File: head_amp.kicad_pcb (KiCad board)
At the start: 2 copper layers, 42 x 64.5 mm, 26 parts, among them J1 Conn_01x02, J2 Headset Port, J3 Ear Mic Input, J4 Speaker Output, SW1 SW_Wuerth_450301014042, U1 LM124DR

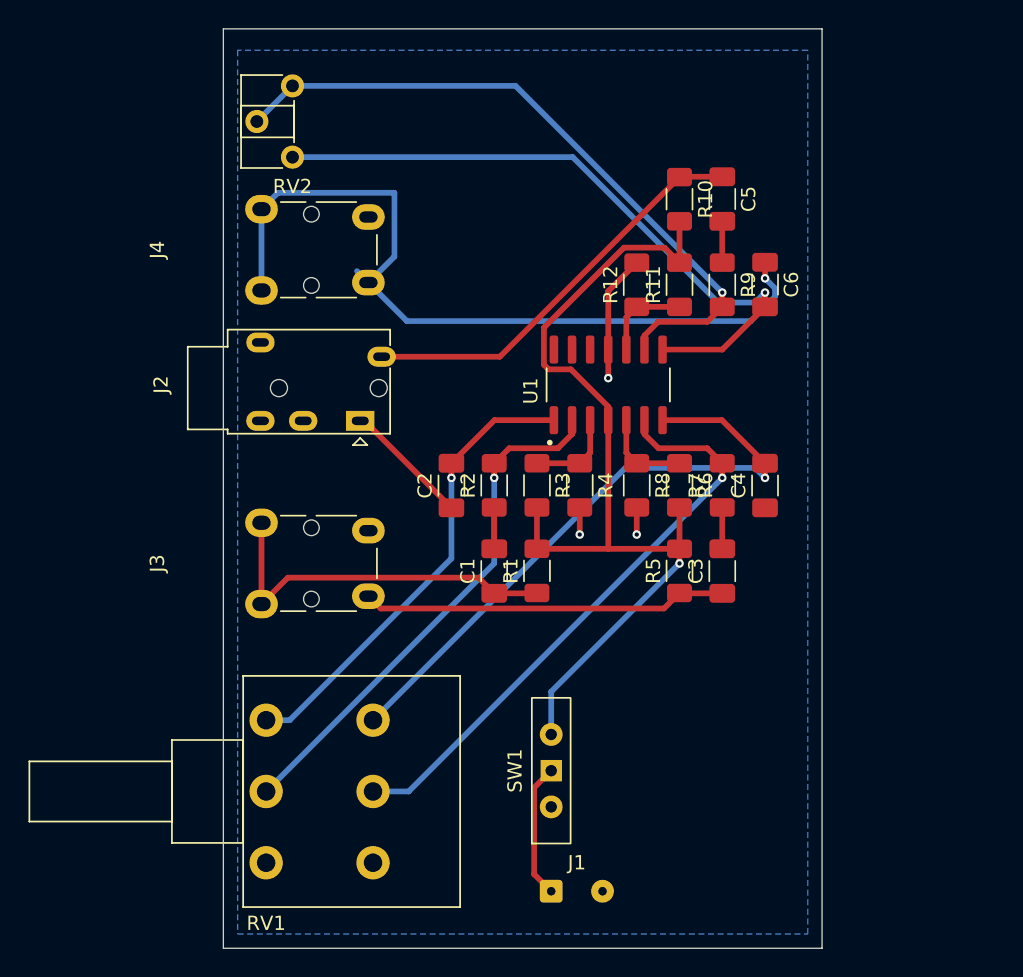
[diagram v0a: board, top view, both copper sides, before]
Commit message: Route PCB :3
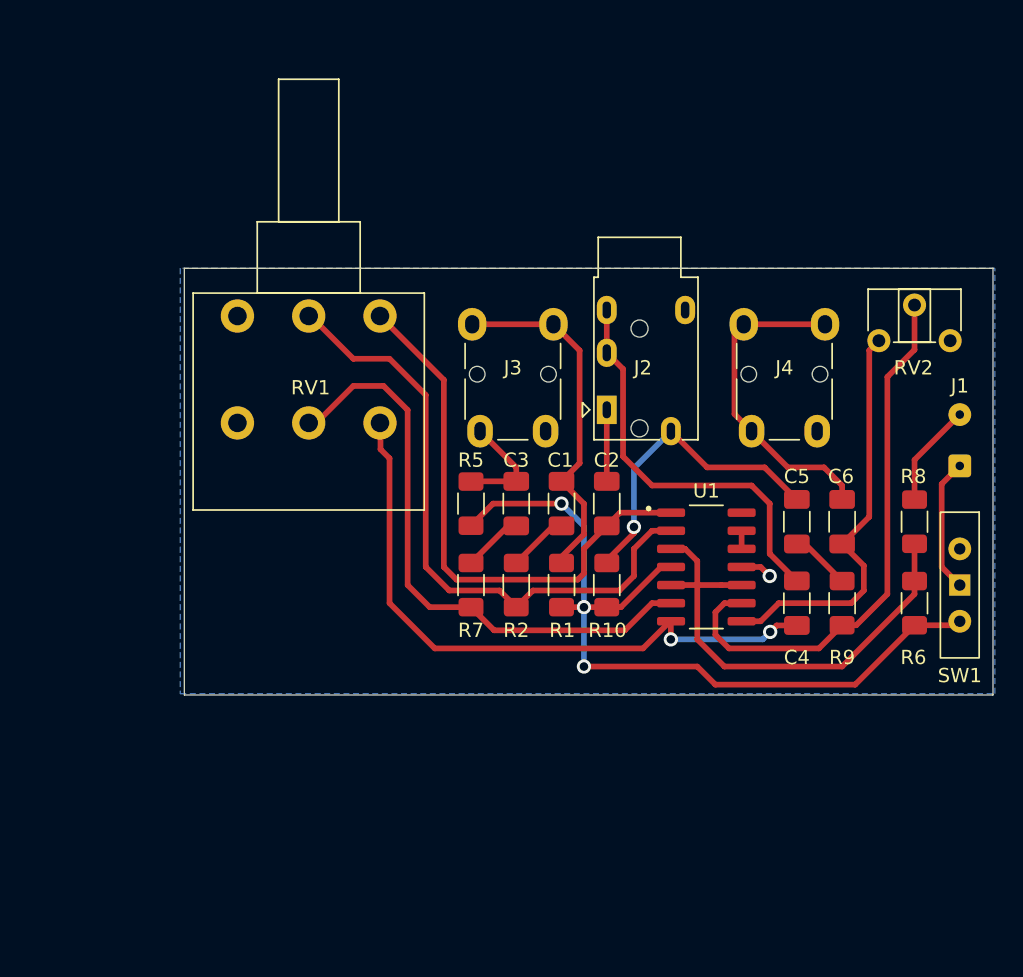
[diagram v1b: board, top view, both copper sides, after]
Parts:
- removed R11, R12, R3, R4: 10k, Resistor_SMD:R_1206_3216Metric_Pad1.30x1.75mm_HandSolder
- moved RV2 43.1 mm to (103.0, 79.4), turned to 90 degrees
- moved J1 41.4 mm to (108.7, 88.2), turned to 90 degrees
- moved J4 33.9 mm to (93.5, 78.2), turned to 0 degrees
- moved SW1 31.5 mm to (108.7, 96.5), turned to -90 degrees
- moved RV1 29.5 mm to (68.0, 77.6), turned to 90 degrees
- moved R10 27.5 mm to (83.9, 96.5)
- moved J3 24.6 mm to (74.5, 78.2), turned to 0 degrees
- moved R9 23.9 mm to (100.4, 97.8)
- moved C5 23.2 mm to (97.2, 92.1)
- moved R8 19.7 mm to (105.5, 92.1), turned to 90 degrees
- moved R7 19.0 mm to (74.4, 96.5), turned to -90 degrees
- moved R6 18.4 mm to (105.5, 97.8)
- moved C6 17.5 mm to (100.4, 92.1)
- moved J2 17.3 mm to (83.9, 84.2), turned to 0 degrees
- moved R5 15.4 mm to (74.4, 90.8), turned to -90 degrees
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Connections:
- J2 pad R1: (no net) -> Net-(C4-Pad1)
- J2 pad R2: (no net) -> Net-(C4-Pad1)
- R6 pad 1: Net-(U1B-+) -> VRef
- R8 pad 1: Net-(U1B-+) -> VRef
- RV2 pad 3: Net-(U1C--) -> unconnected-(RV2-Pad3)
- U1 pad 10: Net-(U1C-+) -> VRef
- U1 pad 12: unconnected-(U1D-+-Pad12) -> Net-(U1D-+)
- U1 pad 13: unconnected-(U1D---Pad13) -> Net-(U1D-+)
- U1 pad 3: Net-(U1A-+) -> VRef
- U1 pad 5: Net-(U1B-+) -> VRef
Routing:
- net VRef: track 0.00 -> 35.0 mm
- net Net-(C6-Pad1): track 56.7 -> 22.9 mm, vias 1 -> 0
- net Net-(C4-Pad1): track 0.00 -> 28.6 mm
- net Net-(C6-Pad2): track 47.1 -> 28.7 mm, vias 1 -> 0
- net Net-(C3-Pad1): track 25.6 -> 7.75 mm
- net Vdd: track 66.0 -> 56.7 mm, vias 1 -> 3
- net Net-(U1C--): track 48.0 -> 38.8 mm, vias 1 -> 0
- net Net-(U1A--): track 36.9 -> 44.3 mm, vias 1 -> 0
- net Net-(C5-Pad1): track 29.1 -> 22.2 mm, vias 0 -> 1
- net Net-(U1B-+): track 6.33 -> 0.00 mm
- net Net-(U1A-+): track 6.33 -> 0.00 mm
- net Net-(U1C-+): track 6.30 -> 0.00 mm
- net Net-(C2-Pad2): track 32.8 -> 38.7 mm, vias 1 -> 0
- net Net-(C2-Pad1): track 8.93 -> 5.02 mm
- net GND: track 12.7 -> 9.51 mm, vias 3 -> 1
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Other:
- board size 42 x 64.5 mm -> 56.7 x 29.9 mm
